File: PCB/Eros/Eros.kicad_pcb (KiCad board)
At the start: 2 copper layers, 72.2 x 80.5 mm, 107 parts, among them J1 USB_C_PowerOnly_6P, J2 UART, J3 Li-ion, J4 Conn_01x08_Socket, J5 Conn_01x03_Socket, J6 Micro_SD_Card, J7 AudioJack3, Q1 BC817, SW1 SW_Push, SW2 SW_Push, SW3 SW_Push, SW4 SW_Push, SW5 SW_Push, SW6 SW_SPDT, U1 ESP32-WROOM-32E, U2 LIS3DH, U3 MCP73831-2-OT, U4 AP2112K-3.3, U5 ADS1115IDGS, U6 MCP100-315D, U7 AD8232, U8 OPA333xxD

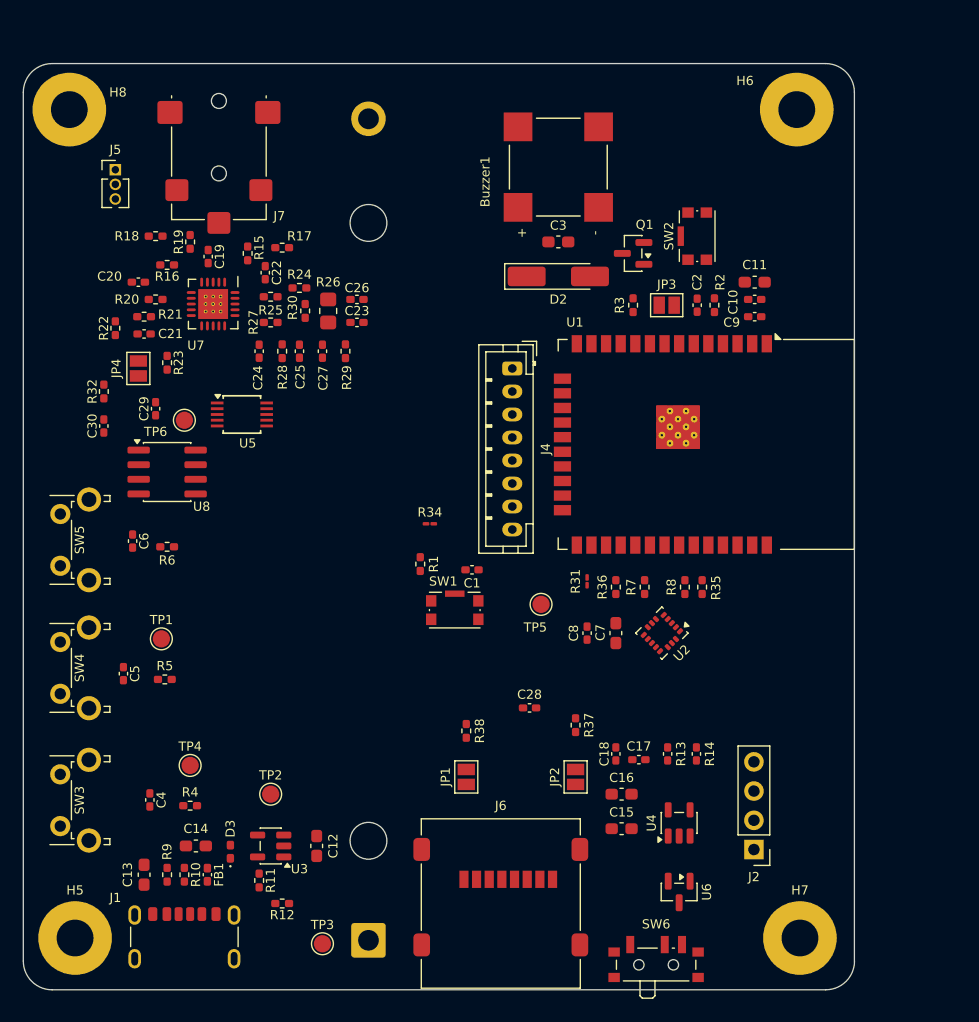
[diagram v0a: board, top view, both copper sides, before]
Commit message: Poprawa schematu oraz ulozenie komponentow
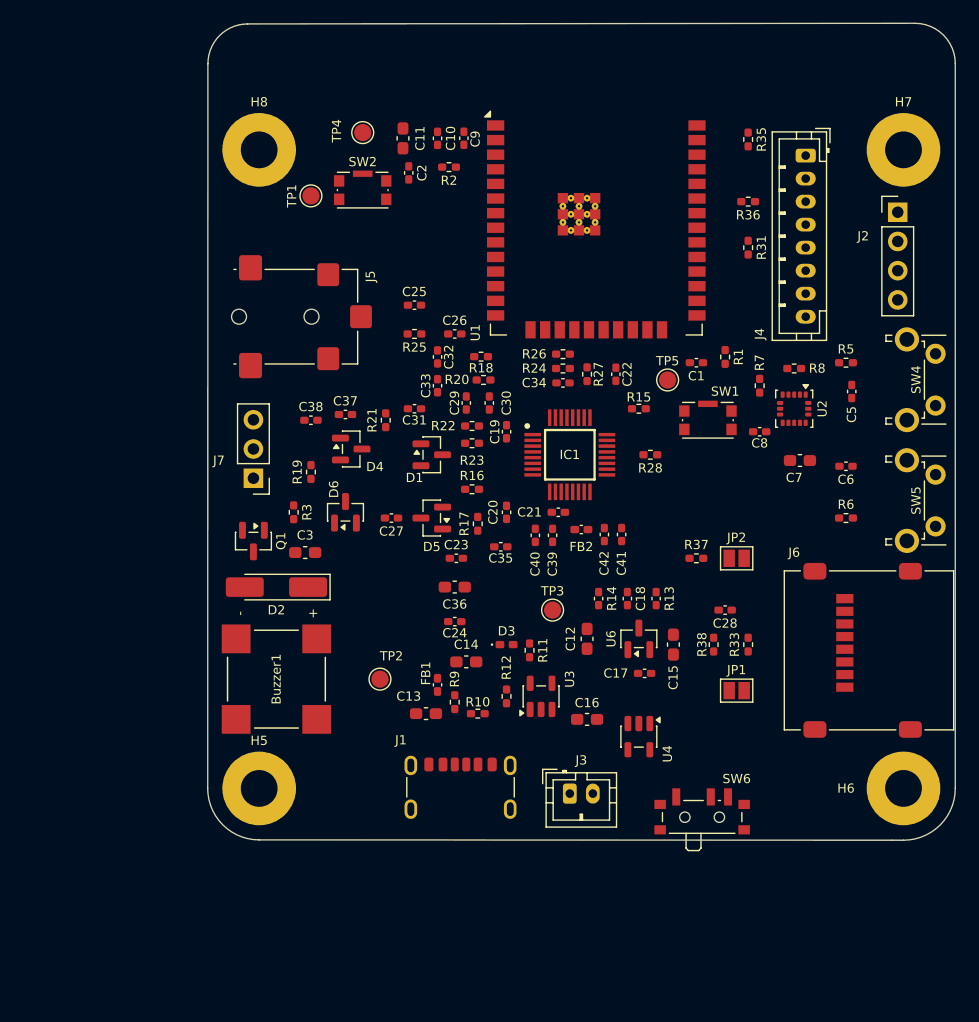
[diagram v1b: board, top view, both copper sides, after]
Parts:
- removed C4: 100n, Capacitor_SMD:C_0402_1005Metric_Pad0.74x0.62mm_HandSolder
- removed JP3, JP4: SolderJumper_2_Open, Jumper:SolderJumper-2_P1.3mm_Open_Pad1.0x1.5mm
- removed R29, R30: R, Resistor_SMD:R_0402_1005Metric_Pad0.72x0.64mm_HandSolder
- removed R32, R4: 10k, Resistor_SMD:R_0402_1005Metric_Pad0.72x0.64mm_HandSolder
- removed R34: 10k, Resistor_SMD:R_01005_0402Metric_Pad0.57x0.30mm_HandSolder
- removed SW3: SW_Push, Button_Switch_THT:SW_Tactile_SPST_Angled_PTS645Vx39-2LFS
- removed TP6: TestPoint, TestPoint:TestPoint_Pad_D1.5mm
- removed U5: ADS1115IDGS, Package_SO:TSSOP-10_3x3mm_P0.5mm
- removed U7: AD8232, AD8232:QFN-20_EP_4x4_Pitch0.5mm
- removed U8: OPA333xxD, Package_SO:SOIC-8_3.9x4.9mm_P1.27mm
- added C31: 100n, Capacitor_SMD:C_0402_1005Metric_Pad0.74x0.62mm_HandSolder, F.Cu at (170.5, 83.0)
- added C32: 1n, Capacitor_SMD:C_0402_1005Metric_Pad0.74x0.62mm_HandSolder, F.Cu at (172.5, 78.5)
- added C33: 1n, Capacitor_SMD:C_0402_1005Metric_Pad0.74x0.62mm_HandSolder, F.Cu at (172.5, 81.0)
- added C34: 1.5n, Capacitor_SMD:C_0402_1005Metric_Pad0.74x0.62mm_HandSolder, F.Cu at (183.4, 80.8)
- added C35: 100n, Capacitor_SMD:C_0402_1005Metric_Pad0.74x0.62mm_HandSolder, F.Cu at (178.0, 95.0)
- added C36: 10u, Capacitor_SMD:C_0603_1608Metric_Pad1.08x0.95mm_HandSolder, F.Cu at (174.0, 98.5)
- added C37: 47p, Capacitor_SMD:C_0402_1005Metric_Pad0.74x0.62mm_HandSolder, F.Cu at (164.5, 83.5)
- added C38: 47p, Capacitor_SMD:C_0402_1005Metric_Pad0.74x0.62mm_HandSolder, F.Cu at (161.5, 84.0)
- added C39: 100n, Capacitor_SMD:C_0402_1005Metric_Pad0.74x0.62mm_HandSolder, F.Cu at (182.5, 94.0)
- added C40: 1u, Capacitor_SMD:C_0402_1005Metric_Pad0.74x0.62mm_HandSolder, F.Cu at (181.0, 94.0)
- added C41: 100n, Capacitor_SMD:C_0402_1005Metric_Pad0.74x0.62mm_HandSolder, F.Cu at (188.5, 93.9)
- added C42: 1u, Capacitor_SMD:C_0402_1005Metric_Pad0.74x0.62mm_HandSolder, F.Cu at (187.0, 93.9)
- added D1: BAV99, Package_TO_SOT_SMD:SOT-23, F.Cu at (172.0, 87.0)
- added D4: BAV99, Package_TO_SOT_SMD:SOT-23, F.Cu at (165.0, 86.5)
- added D5: BAV99, Package_TO_SOT_SMD:SOT-23, F.Cu at (172.0, 92.5)
- added D6: BAV99, Package_TO_SOT_SMD:SOT-23, F.Cu at (164.5, 92.0)
- added FB2: FerriteBead(600om), Inductor_SMD:L_0402_1005Metric_Pad0.77x0.64mm_HandSolder, F.Cu at (185.0, 93.5)
- added IC1: ADS1292RIPBS, ADS1292:QFP50P700X700X120-32N, F.Cu at (184.0, 87.0)
- added R33: 10k, Resistor_SMD:R_0402_1005Metric_Pad0.72x0.64mm_HandSolder, F.Cu at (199.5, 103.5)
- C19: value 1n -> 47n
- C20: value 10n -> 47n
- C21: value 1.5n -> 2.2u
- C22: value 0.33u -> 2.2u
- C23: value 0.33u -> 22u
- C26, C27: value C -> 2.2n
- C29, C30: value 100n -> 2.2n
- FB1: value FerriteBead -> FerriteBead(120om)
- J3: footprint BHC-18650-1P COMF:BatteryHolder_MPD_BH-18650-PC -> Connector_JST:JST_PH_B2B-PH-K_1x02_P2.00mm_Vertical; moved to F.Cu
- J5: value Conn_01x03_Socket -> AudioJack3; footprint Connector_PinHeader_1.27mm:PinHeader_1x03_P1.27mm_Vertical -> Connector_Audio:Jack_3.5mm_Lumberg_1503_03_Horizontal
- J7: value AudioJack3 -> Conn_01x03_Socket; footprint Connector_Audio:Jack_3.5mm_Lumberg_1503_03_Horizontal -> Connector_PinHeader_2.54mm:PinHeader_1x03_P2.54mm_Vertical
- R15: value 180k -> 10k
- R16: value 180k -> 10M
- R18: value 10M -> 40.2k
- R19: value 360k -> 51k
- R20: value 100k -> 40.2k
- R21: value 1M -> 51k
- R22, R23: value 1M -> 10M
- R24: value 10M -> 1M
- R25, R27: value 10M -> 100k
- R26: value 1.4M -> 0R; footprint Resistor_SMD:R_0805_2012Metric_Pad1.20x1.40mm_HandSolder -> Resistor_SMD:R_0402_1005Metric_Pad0.72x0.64mm_HandSolder
- R28: value 10M -> 10k
- R31: footprint Resistor_SMD:R_01005_0402Metric_Pad0.57x0.30mm_HandSolder -> Resistor_SMD:R_0402_1005Metric_Pad0.72x0.64mm_HandSolder
- U1: footprint RF_Module:ESP32-WROOM-32D -> RF_Module:ESP32-WROOM-32E
- moved SW4 81.6 mm to (215.8, 78.2), turned to -90 degrees
- moved SW5 76.5 mm to (215.8, 88.7), turned to -90 degrees
- moved H7 69.1 mm to (213.0, 60.5)
- moved C5 67.9 mm to (208.5, 81.5), turned to -90 degrees
- moved R5 65.3 mm to (208.0, 79.0)
- moved C6 62.3 mm to (208.0, 88.0), turned to 180 degrees
- moved H6 59.7 mm to (213.0, 116.0)
- moved R6 59.1 mm to (208.0, 92.5), turned to 0 degrees
- moved TP4 57.0 mm to (166.0, 59.0), turned to 90 degrees
- moved J2 56.8 mm to (212.5, 65.9), turned to 0 degrees
- moved Buzzer1 50.8 mm to (158.5, 106.5), turned to -90 degrees
- moved Q1 41.4 mm to (156.5, 94.5), turned to -90 degrees
- moved TP1 40.6 mm to (161.5, 64.5), turned to 90 degrees
- moved C21 39.2 mm to (183.0, 92.0)
- moved R35 39.1 mm to (199.5, 59.6), turned to -90 degrees
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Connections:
- Buzzer1 pad P: VS -> +3.3V
- C10 pad 2: VS -> +3.3V
- C11 pad 2: VS -> +3.3V
- C16 pad 2: VS -> +3.3V
- C18 pad 1: ADC1 -> ADC
- C19 pad 2: Net-(U7-RLD) -> Net-(IC1-PGA1N)
- C20 pad 1: OPAMP+ -> Net-(IC1-PGA2P)
- C20 pad 2: REFOUT -> Net-(IC1-PGA2N)
- C21 pad 1: Net-(C21-Pad1) -> VCAP1
- C21 pad 2: OUTPUT -> GND
- C22 pad 1: Net-(U7-HPDRIVE) -> VCAP2
- C22 pad 2: Net-(U7-HPSENSE) -> GND
- C23 pad 1: SW -> VREFP
- C23 pad 2: REFOUT -> GND
- C24 pad 1: GND -> VREFP
- C24 pad 2: VS -> GND
- C25 pad 1: GND -> LA
- C25 pad 2: REFIN -> Net-(C25-Pad2)
- C26 pad 1: SW -> Net-(C25-Pad2)
- C26 pad 2: REFOUT -> Net-(C26-Pad2)
- C27 pad 1: GND -> IN1P
- C27 pad 2: REFIN -> Net-(C25-Pad2)
- C28 pad 1: VS -> +3.3V
- C29 pad 1: VS -> Net-(C29-Pad1)
- C29 pad 2: GND -> Net-(C29-Pad2)
- C3 pad 1: VS -> +3.3V
- C30 pad 1: Net-(U8-+) -> IN1N
- C30 pad 2: GND -> Net-(C29-Pad1)
- C7 pad 2: VS -> +3.3V
- C8 pad 2: VS -> +3.3V
- C9 pad 2: VS -> +3.3V
- D2 pad 1: VS -> +3.3V
- J2 pad 1: VS -> +3.3V
- J4 pad 1: VS -> +3.3V
- J4 pad 3: HSPI_MOSI -> VSPI_MOSI
- J4 pad 4: HSPI_CLK -> VSPI_SCK
- J4 pad 5: HSPI_CS -> DISP_CS
- J6 pad 4: VS -> +3.3V
- R1 pad 1: VS -> +3.3V
- R13 pad 1: ADC1 -> ADC
- R14 pad 1: ADC1 -> ADC
- R15 pad 1: LA -> +3.3V
- R15 pad 2: Net-(U7-+IN) -> HSPI_CS
- R16 pad 1: RA -> AVDD
- R16 pad 2: Net-(U7--IN) -> IN1P
- R17 pad 1: LA -> GND
- R17 pad 2: VS -> IN1P
- R18 pad 1: VS -> Net-(C26-Pad2)
- R18 pad 2: RA -> IN3P
- R19 pad 1: RL -> IN2P
- R19 pad 2: Net-(U7-RLD) -> LA
- R2 pad 1: VS -> +3.3V
- R20 pad 1: OPAMP- -> Net-(C29-Pad2)
- R20 pad 2: REFOUT -> IN3N
- R21 pad 1: OPAMP- -> IN2N
- R21 pad 2: OUTPUT -> RA
- R22 pad 1: Net-(C21-Pad1) -> GND
- R22 pad 2: OPAMP+ -> IN1N
- R23 pad 1: IAOUT -> AVDD
- R23 pad 2: Net-(C21-Pad1) -> IN1N
- R24 pad 1: Net-(U7-HPSENSE) -> RLDINV
- R24 pad 2: Net-(R24-Pad2) -> RLDOUT
- R25 pad 1: Net-(R24-Pad2) -> RLDINV
- R25 pad 2: IAOUT -> RL
- R26 pad 1: SW -> RLDINV
- R26 pad 2: Net-(R24-Pad2) -> RLDOUT
- R27 pad 1: REFIN -> RLDIN
- R27 pad 2: VS -> RLDINV
- R28 pad 1: REFIN -> GND
- R28 pad 2: GND -> HSPI_SCK
- R31 pad 1: VS -> +3.3V
- R31 pad 2: VSPI_CS -> DISP_CS
- R35 pad 1: VS -> +3.3V
- R36 pad 1: VS -> +3.3V
- R37 pad 1: VS -> +3.3V
- R38 pad 1: VS -> +3.3V
- R5 pad 1: VS -> +3.3V
- R6 pad 1: VS -> +3.3V
- R7 pad 1: VS -> +3.3V
- R8 pad 1: VS -> +3.3V
- TP4 pad 1: VS -> +3.3V
- U1 pad 10: BUTTON_1 -> START
- U1 pad 11: BUTTON_2 -> PWDN
- U1 pad 12: BUTTON_3 -> BUZZER
- U1 pad 13: HSPI_CLK -> HSPI_MISO
- U1 pad 14: LOD+ -> HSPI_SCK
- U1 pad 2: VS -> +3.3V
- U1 pad 29: VSPI_CS -> DISP_CS
- U1 pad 4: Net-(JP3-B) -> ADC
- U1 pad 5: unconnected-(U1-SENSOR_VN-Pad5) -> BUTTON_2
- U1 pad 6: LOD- -> DRDY
- U1 pad 7: BUZZER -> BUTTON_1
- U1 pad 8: SDN -> VSPI_CS
- U2 pad 1: VS -> +3.3V
- U2 pad 14: VS -> +3.3V
- U2 pad 8: VS -> +3.3V
- U4 pad 5: VS -> +3.3V
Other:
- board size 72.2 x 80.5 mm -> 65 x 71 mm
